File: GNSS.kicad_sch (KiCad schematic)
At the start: 10 parts, among them J3 Conn_Coaxial, J9 Conn_01x02_Pin, U5 NEO-M9N

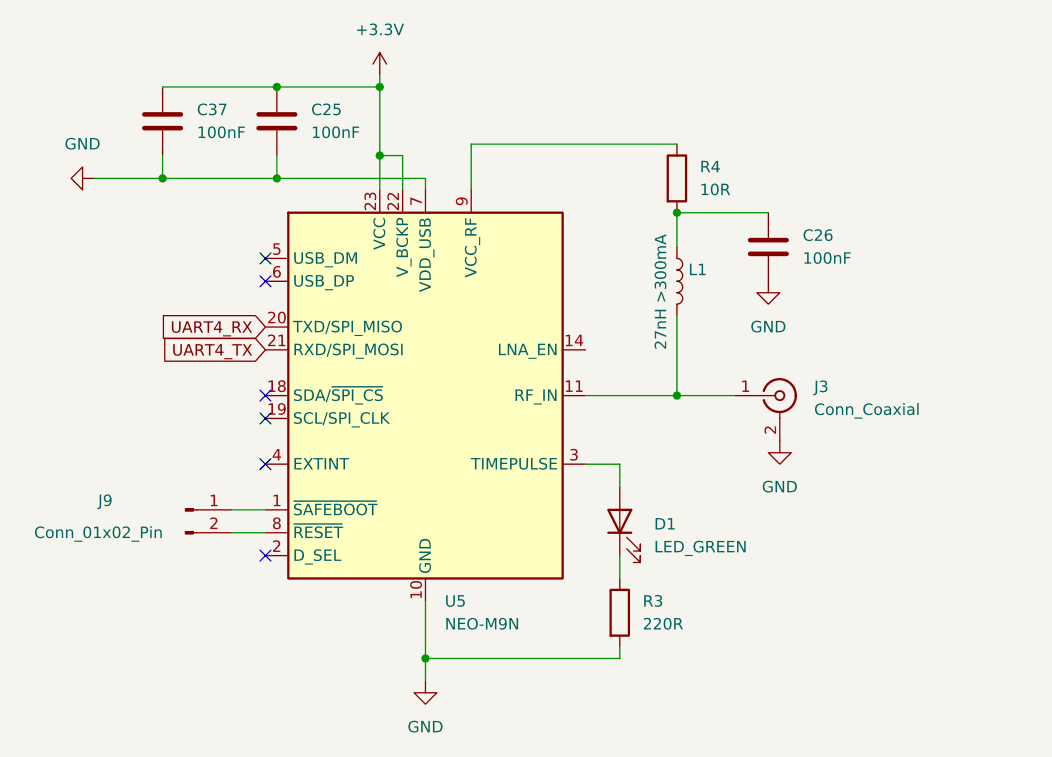
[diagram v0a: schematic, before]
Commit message: Update PCB
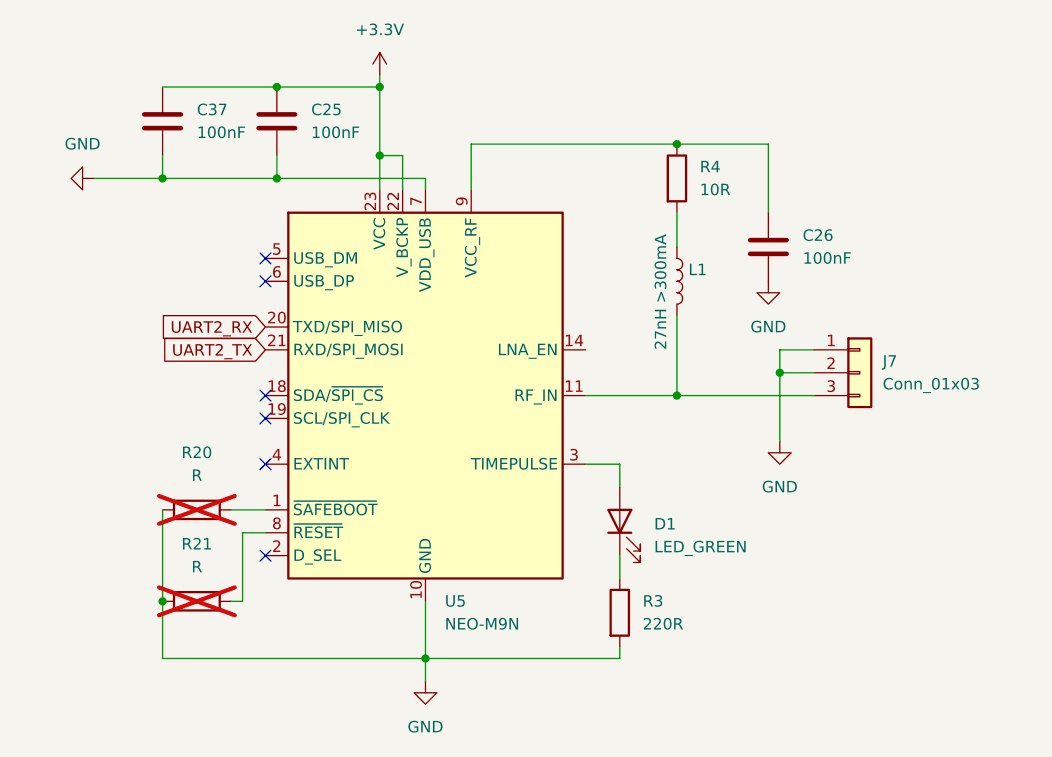
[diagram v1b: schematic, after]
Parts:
- removed J3: Conn_Coaxial, Connector_Coaxial:BNC_Amphenol_B6252HB-NPP3G-50_Horizontal, symbol Connector:Conn_Coaxial
- removed J9: Conn_01x02_Pin, Connector_PinHeader_2.54mm:PinHeader_1x02_P2.54mm_Vertical, symbol Connector:Conn_01x02_Pin
- added J7: Conn_01x03, dep:CONSMA001SMDG, symbol Connector_Generic:Conn_01x03
- added R20, R21: R, Resistor_SMD:R_0402_1005Metric, symbol Device:R
- R4: footprint Resistor_SMD:R_0402_1005Metric -> Resistor_SMD:R_0603_1608Metric
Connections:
- net GND: now also J7.1 (Pin_1), J7.2 (Pin_2), R20.2, R21.2
- net at U5.1 (~{SAFEBOOT}): now also R20.1
- net at L1.2, U5.11 (RF_IN): now also J7.3 (Pin_3)
- net at U5.8 (~{RESET}): now also R21.1
- net at R4.1, U5.9 (VCC_RF): now also C26.1
- net at L1.1, R4.2: no longer C26.1
- net UART4_RX renamed UART2_RX
- net UART4_TX renamed UART2_TX

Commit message: questionable changes
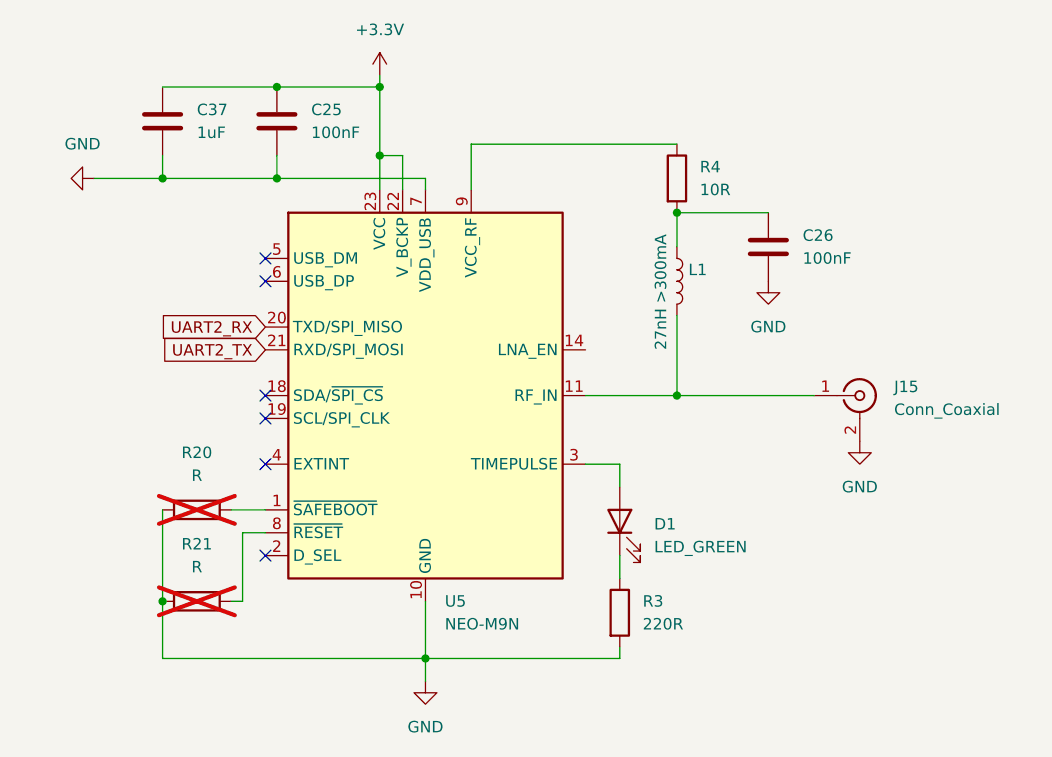
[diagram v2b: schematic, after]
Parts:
- removed J7: Conn_01x03, dep:CONSMA001SMDG, symbol Connector_Generic:Conn_01x03
- added J15: Conn_Coaxial, Connector_Coaxial:U.FL_Hirose_U.FL-R-SMT-1_Vertical, symbol Connector:Conn_Coaxial
- C37: value 100nF -> 1uF
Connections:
- net GND: now also J15.2 (Ext)
- net at L1.2, U5.11 (RF_IN): now also J15.1 (In)
- net at R4.1, U5.9 (VCC_RF): no longer C26.1
- net at L1.1, R4.2: now also C26.1
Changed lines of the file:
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@@
 	(paper "A4")
-	(junction
-		(at 177.8 92.71)
-		(diameter 0)
-		(color 0 0 0 0)
-	)
 	(junction
 		(at 109.22 118.11)
@@
 	)
 	(junction
-		(at 166.37 67.31)
-		(diameter 0)
-		(color 0 0 0 0)
-	)
-	(junction
 		(at 109.22 71.12)
 		(diameter 0)
@@
 		(color 0 0 0 0)
 	)
+	(junction
+		(at 166.37 74.93)
+		(diameter 0)
+		(color 0 0 0 0)
+	)
 	(no_connect
 		(at 120.65 95.25)
@@
 	(wire
 		(pts
-			(xy 177.8 92.71) (xy 181.61 92.71)
-		)
-		(stroke
-			(width 0)
-			(type default)
-		)
-	)
-	(wire
-		(pts
 			(xy 166.37 95.25) (xy 181.61 95.25)
 		)
@@
 	(wire
 		(pts
-			(xy 177.8 100.33) (xy 177.8 92.71)
-		)
-		(stroke
-			(width 0)
-			(type default)
-		)
-	)
-	(wire
-		(pts
 			(xy 118.11 118.11) (xy 118.11 110.49)
 		)
@@
 	(wire
 		(pts
-			(xy 177.8 90.17) (xy 181.61 90.17)
-		)
-		(stroke
-			(width 0)
-			(type default)
-		)
-	)
-	(wire
-		(pts
 			(xy 135.89 72.39) (xy 135.89 68.58)
 		)
@@
 	(wire
 		(pts
-			(xy 177.8 92.71) (xy 177.8 90.17)
-		)
-		(stroke
-			(width 0)
-			(type default)
-		)
-	)
-	(wire
-		(pts
-			(xy 176.53 67.31) (xy 176.53 74.93)
-		)
-		(stroke
-			(width 0)
-			(type default)
-		)
-	)
-	(wire
-		(pts
 			(xy 109.22 124.46) (xy 138.43 124.46)
 		)
@@
 	(wire
 		(pts
-			(xy 166.37 67.31) (xy 176.53 67.31)
+			(xy 166.37 74.93) (xy 176.53 74.93)
 		)
 		(stroke
@@
 	(symbol
 		(lib_id "power:GND")
-		(at 177.8 100.33 0)
+		(at 186.69 100.33 0)
 		(unit 1)
 		(exclude_from_sim no)
@@
 		(fields_autoplaced yes)
 		(property "Reference" "#PWR037"
-			(at 177.8 106.68 0)
+			(at 186.69 106.68 0)
 			(effects
 				(font
@@
 		)
 		(property "Value" "GND"
-			(at 177.8 105.41 0)
+			(at 186.69 105.41 0)
 			(effects
 				(font
@@
 		)
 		(property "Footprint" ""
-			(at 177.8 100.33 0)
+			(at 186.69 100.33 0)
 			(effects
 				(font
@@
 		)
 		(property "Datasheet" ""
-			(at 177.8 100.33 0)
+			(at 186.69 100.33 0)
 			(effects
 				(font
@@
 		)
 		(property "Description" "Power symbol creates a global label with name \"GND\" , ground"
-			(at 177.8 100.33 0)
+			(at 186.69 100.33 0)
 			(effects
 				(font
@@
 			)
 		)
-		(property "Value" "100nF"
+		(property "Value" "1uF"
 			(at 113.03 66.0399 0)
 			(effects
@@
 	)
 	(symbol
-		(lib_id "Connector_Generic:Conn_01x03")
-		(at 186.69 92.71 0)
-		(unit 1)
-		(exclude_from_sim no)
-		(in_bom yes)
-		(on_board yes)
-		(dnp no)
-		(fields_autoplaced yes)
-		(property "Reference" "J7"
-			(at 189.23 91.4399 0)
-			(effects
-				(font
-					(size 1.27 1.27)
-				)
-				(justify left)
-			)
-		)
-		(property "Value" "Conn_01x03"
-			(at 189.23 93.9799 0)
-			(effects
-				(font
-					(size 1.27 1.27)
-				)
-				(justify left)
-			)
-		)
-		(property "Footprint" "dep:CONSMA001SMDG"
-			(at 186.69 92.71 0)
-			(effects
-				(font
-					(size 1.27 1.27)
-				)
-				(hide yes)
-			)
-		)
-		(property "Datasheet" "~"
-			(at 186.69 92.71 0)
-			(effects
-				(font
-					(size 1.27 1.27)
-				)
-				(hide yes)
-			)
-		)
-		(property "Description" "Generic connector, single row, 01x03, script generated (kicad-library-utils/schlib/autogen/connector/)"
-			(at 186.69 92.71 0)
-			(effects
-				(font
-					(size 1.27 1.27)
-				)
-				(hide yes)
-			)
-		)
-		(pin "2"
-		)
-		(pin "1"
-		)
-		(pin "3"
-		)
-		(instances
-			(project ""
-				(path "/aff8106b-a9b7-4e48-85ad-25b2eb3ce379/f42f4972-519d-4306-8fa1-8314a04aa80d"
-					(reference "J7")
-					(unit 1)
-				)
-			)
-		)
-	)
-	(symbol
 		(lib_id "Device:R")
 		(at 166.37 71.12 0)
@@
 					(unit 1)
 				)
+			)
+		)
+	)
+	(symbol
+		(lib_id "Connector:Conn_Coaxial")
+		(at 186.69 95.25 0)
+		(unit 1)
+		(exclude_from_sim no)
+		(in_bom yes)
+		(on_board yes)
+		(dnp no)
+		(fields_autoplaced yes)
+		(property "Reference" "J15"
+			(at 190.5 94.2731 0)
+			(effects
+				(font
+					(size 1.27 1.27)
+				)
+				(justify left)
+			)
+		)
+		(property "Value" "Conn_Coaxial"
+			(at 190.5 96.8131 0)
+			(effects
+				(font
+					(size 1.27 1.27)
+				)
+				(justify left)
+			)
+		)
+		(property "Footprint" "Connector_Coaxial:U.FL_Hirose_U.FL-R-SMT-1_Vertical"
+			(at 186.69 95.25 0)
+			(effects
+				(font
+					(size 1.27 1.27)
+				)
+				(hide yes)
+			)
+		)
+		(property "Datasheet" "~"
+			(at 186.69 95.25 0)
+			(effects
+				(font
+					(size 1.27 1.27)
+				)
+				(hide yes)
+			)
+		)
+		(property "Description" "coaxial connector (BNC, SMA, SMB, SMC, Cinch/RCA, LEMO, ...)"
+			(at 186.69 95.25 0)
+			(effects
+				(font
+					(size 1.27 1.27)
+				)
+				(hide yes)
+			)
+		)
+		(pin "2"
+		)
+		(pin "1"
+		)
+		(instances
+			(project ""
+				(path "/aff8106b-a9b7-4e48-85ad-25b2eb3ce379/f42f4972-519d-4306-8fa1-8314a04aa80d"
+					(reference "J15")
+					(unit 1)
+				)

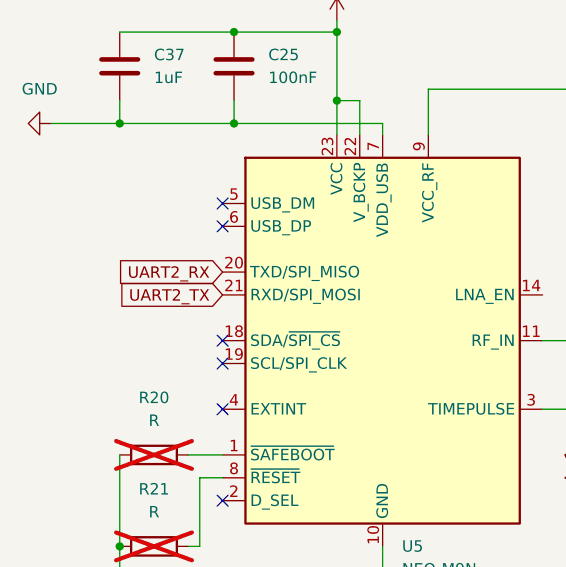
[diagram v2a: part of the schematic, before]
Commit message: PCB Update
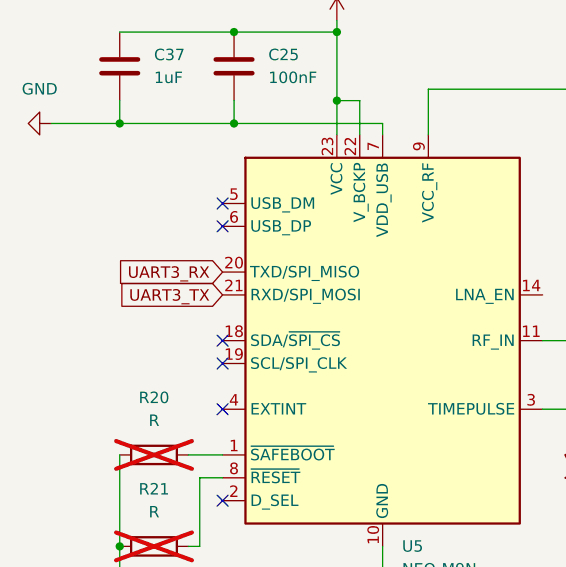
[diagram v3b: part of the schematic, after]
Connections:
- net UART2_RX renamed UART3_RX
- net UART2_TX renamed UART3_TX
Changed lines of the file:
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@@
 		)
 	)
-	(global_label "UART2_TX"
+	(global_label "UART3_TX"
 		(shape input)
 		(at 120.65 90.17 180)
@@
 		)
 	)
-	(global_label "UART2_RX"
+	(global_label "UART3_RX"
 		(shape input)
 		(at 120.65 87.63 180)
